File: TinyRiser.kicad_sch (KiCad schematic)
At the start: 24 parts, among them J2 Bus_PCI_Express_x16, J3 Bus_M.2_Socket_M, J4 fancontrol_header, M1 Fan_4pin

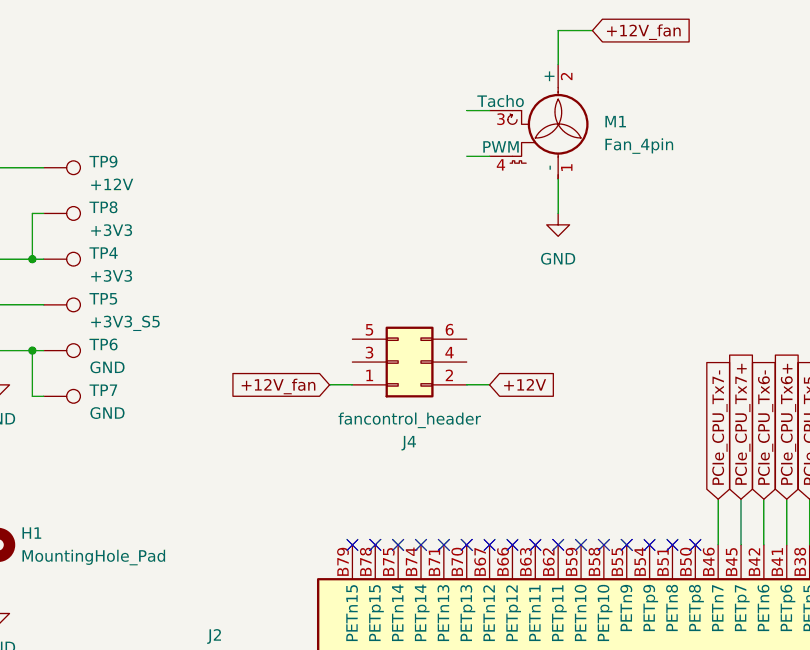
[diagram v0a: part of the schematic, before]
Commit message: Mostly finished fan connector implementation
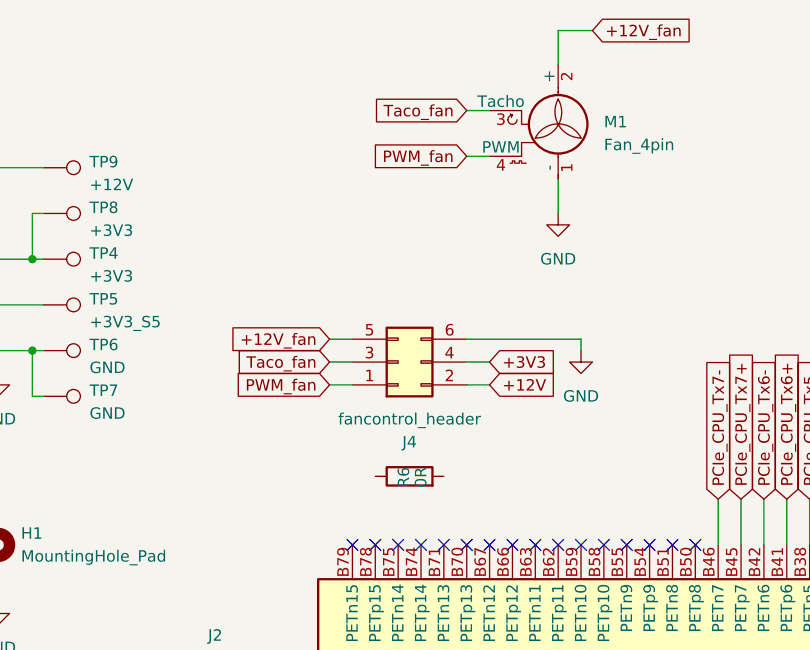
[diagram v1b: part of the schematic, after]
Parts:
- added R6: 0R, Resistor_SMD:R_0603_1608Metric_Pad0.98x0.95mm_HandSolder, symbol Device:R
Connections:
- net +12V_fan: now also J4.5 (Pin_5); no longer J4.1 (Pin_1)
- net +3V3: now also J4.4 (Pin_4)
- net GND: now also J4.6 (Pin_6)
- net Taco_fan: now reaches J4.3 (Pin_3)
- net Taco_fan: now also M1.3 (Tacho)
- net PWM_fan: now reaches M1.4 (PWM)
- net PWM_fan: now also J4.1 (Pin_1)
